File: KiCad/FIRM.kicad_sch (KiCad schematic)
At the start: 56 parts, among them J1 Conn_01x04_Pin, J2 USB_A, J3 Micro_SD_Card_Det2, Q1 AO3401A, U1 STM32F405RGTx, U2 LM2596S-3.3, U6 AP2112K-3.3, U7 W25Q128JVS, X2 32.768khz, Y1 12mhz

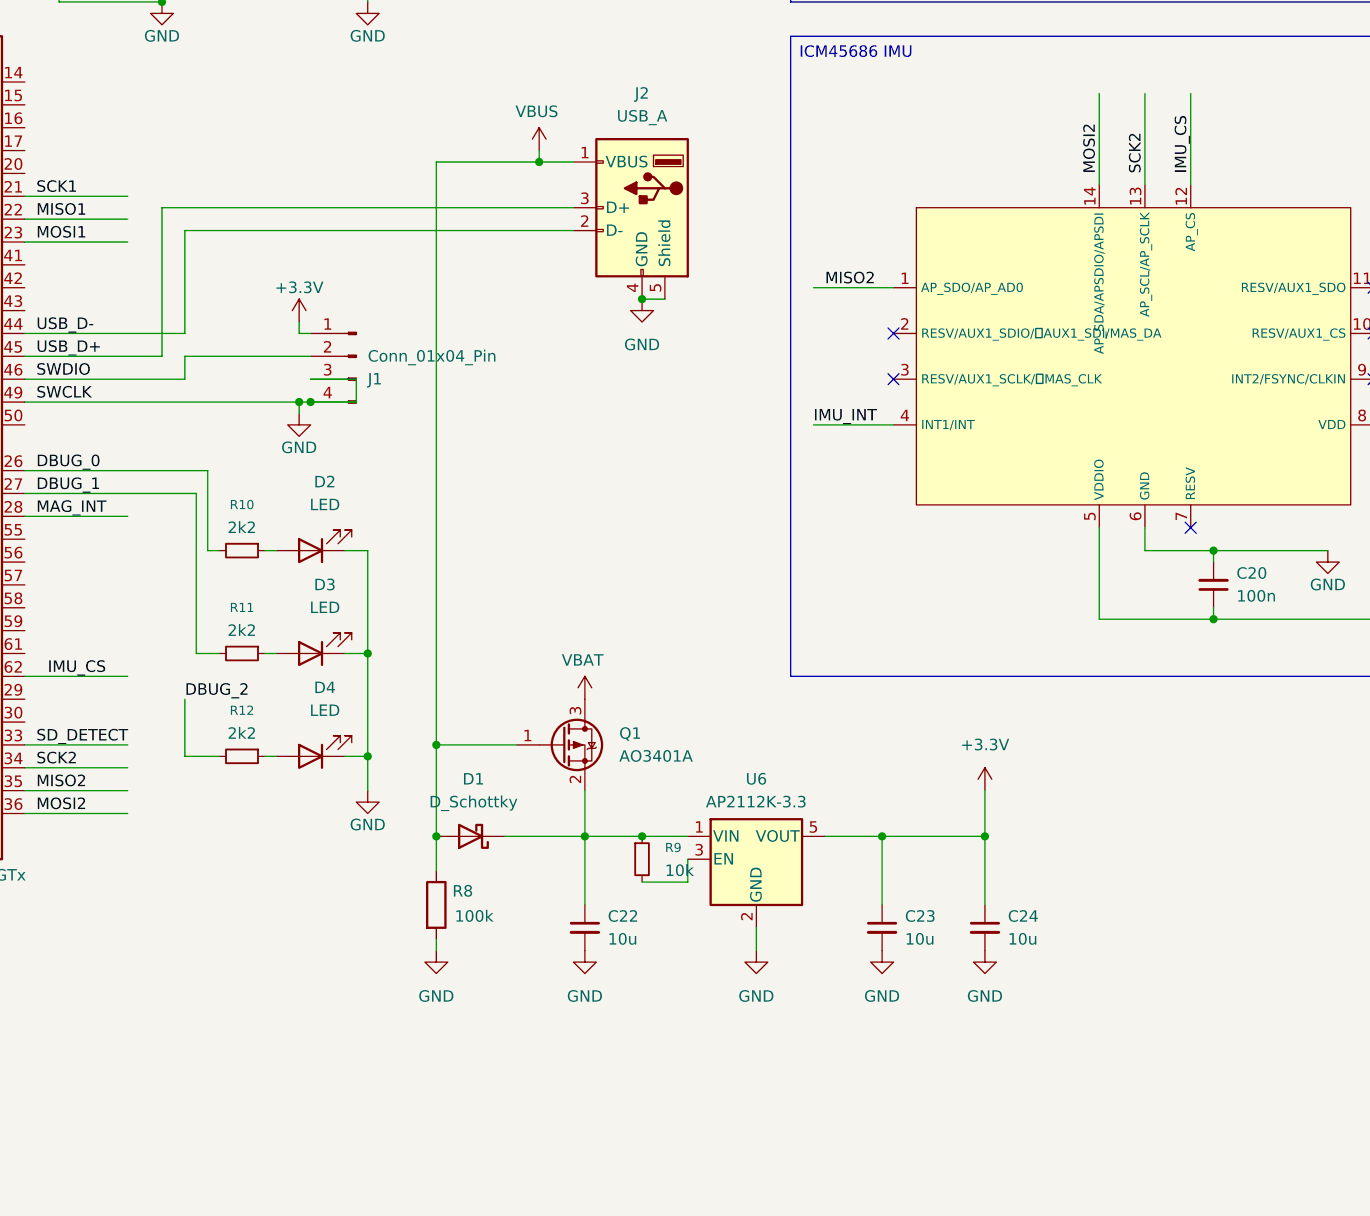
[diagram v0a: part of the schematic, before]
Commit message: test
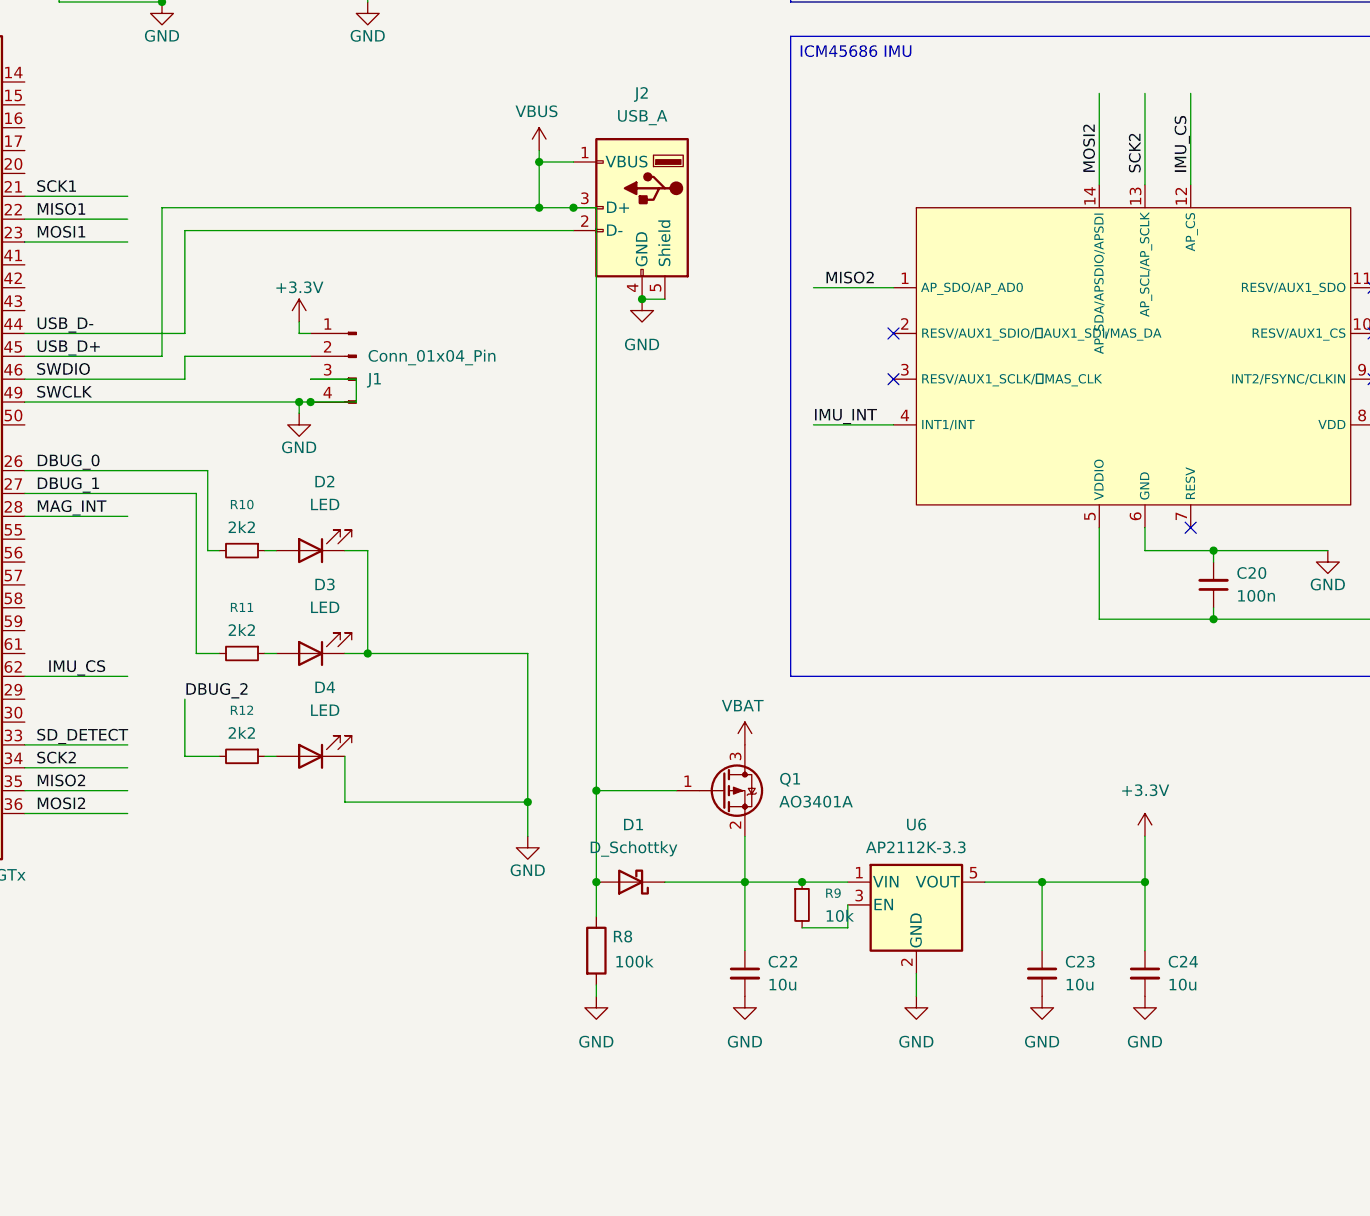
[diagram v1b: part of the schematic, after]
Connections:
- net USB_D+ is gone; now on net VBUS: J2.3 (D+), U1.45 (PA12)
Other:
- moved on the sheet: C22, C23, C24, D1, Q1, R8, R9, U6
